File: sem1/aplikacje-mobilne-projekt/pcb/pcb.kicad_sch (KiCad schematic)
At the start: 26 parts, among them J1 Conn_01x20_Female, J2 Conn_01x20_Female, J3 Conn_01x10_Male, Q1 IRF540N, Q10 IRF540N, Q11 IRF540N, Q12 IRF540N, Q13 IRF540N, Q2 IRF540N, Q3 IRF540N, Q4 IRF540N, Q5 IRF540N, Q6 IRF540N, Q7 IRF540N, Q8 IRF540N, Q9 IRF540N, U1 IRF9540N, U2 IRF9540N, U3 IRF9540N, U4 IRF9540N

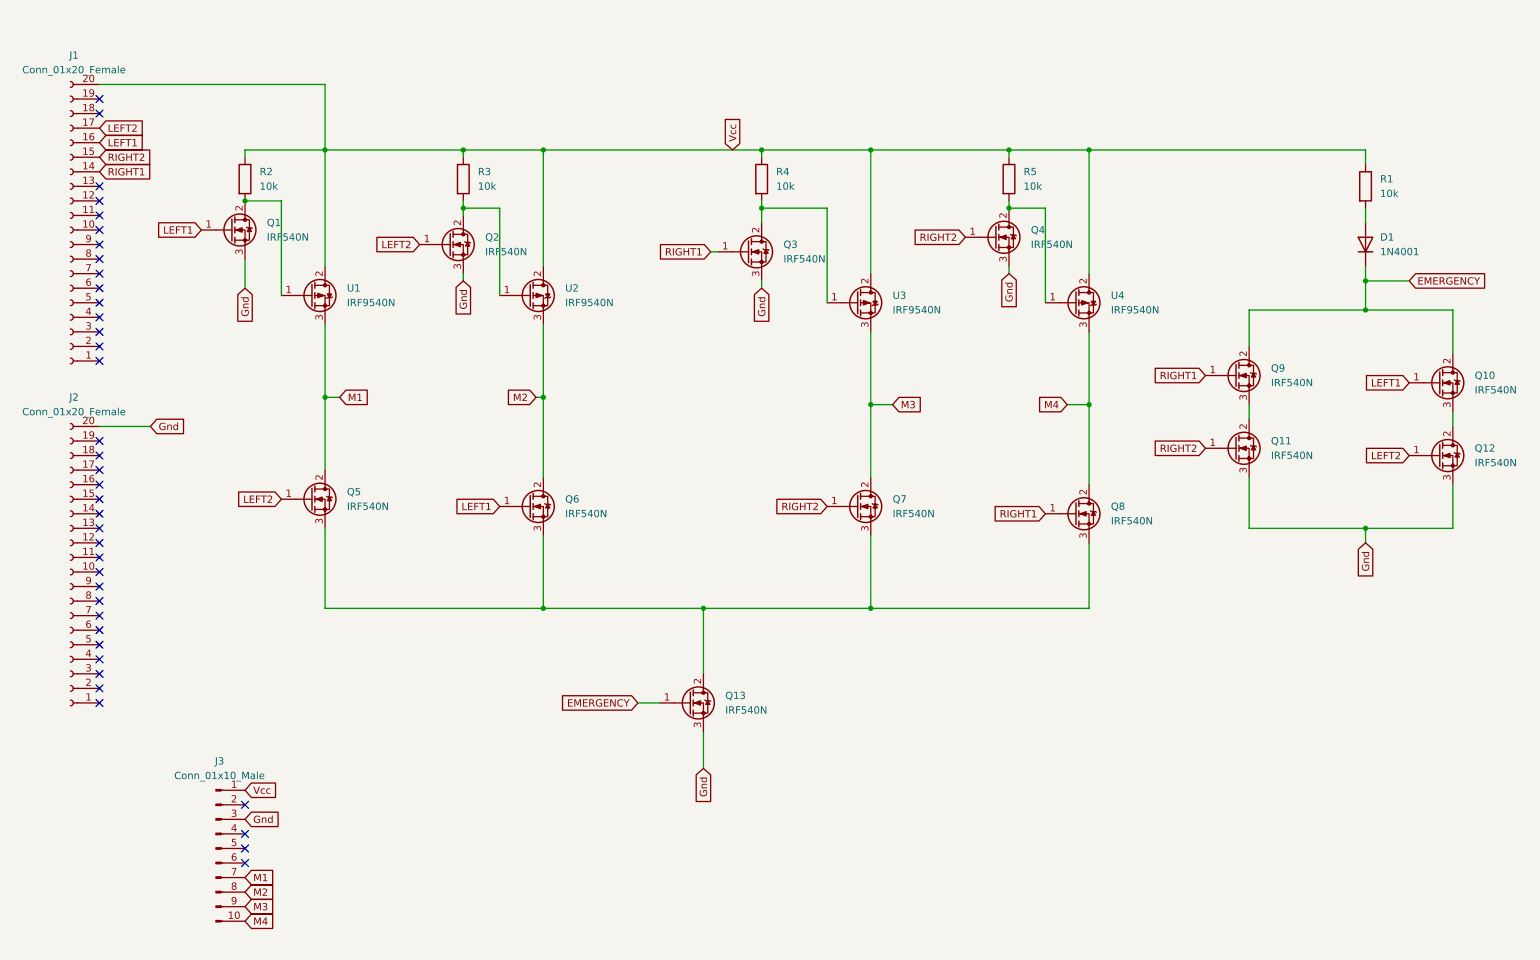
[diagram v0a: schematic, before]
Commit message: this pcb one actually works
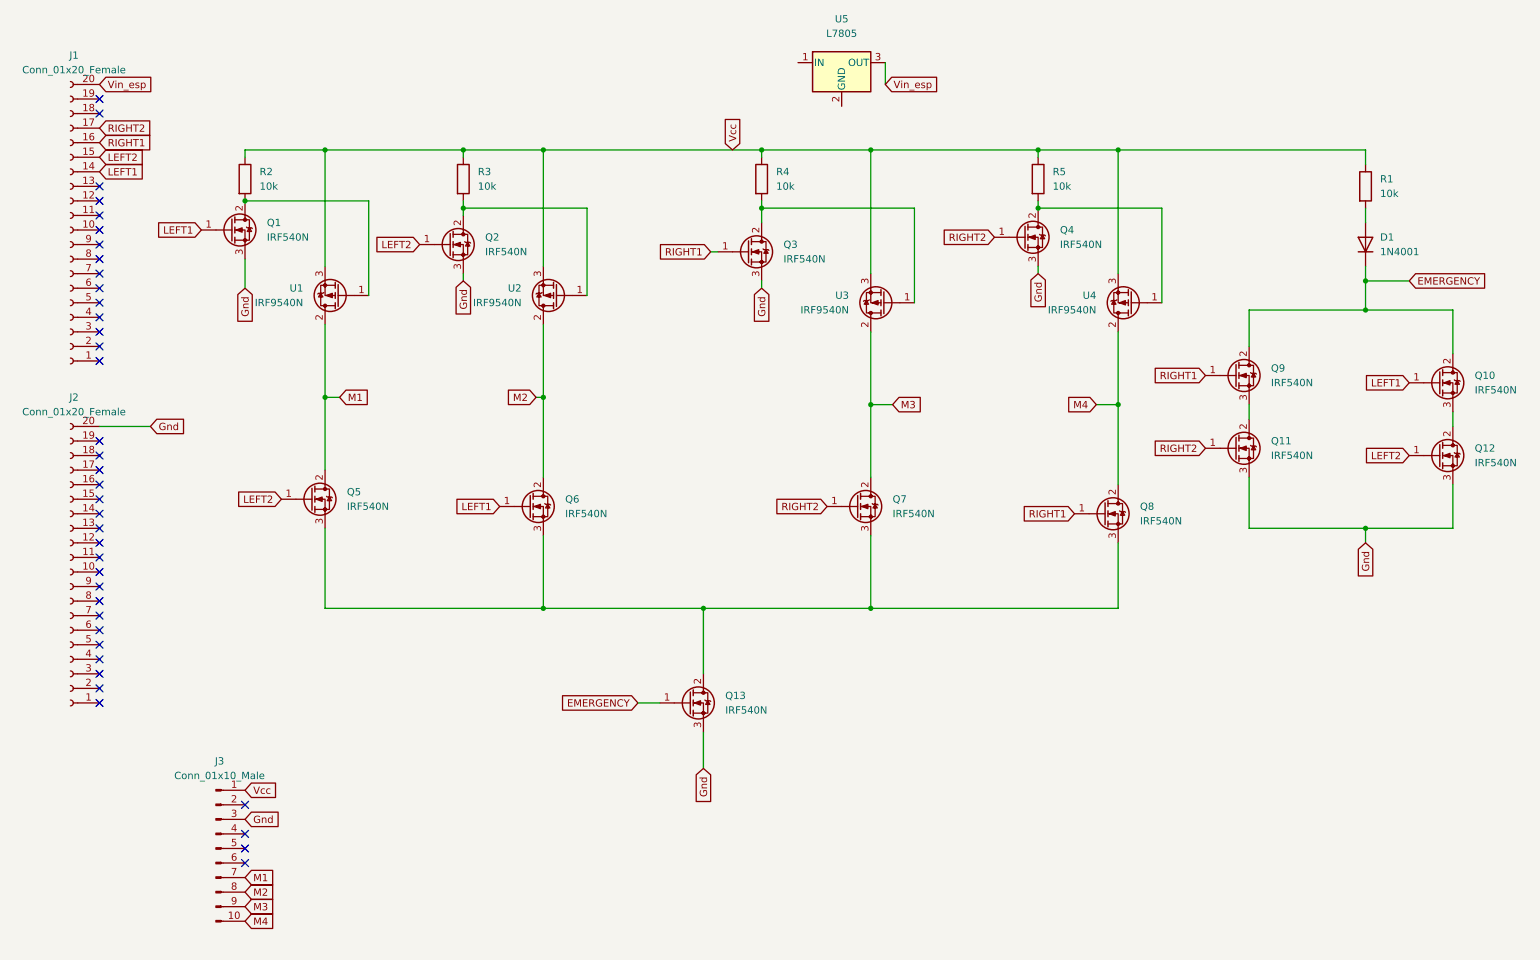
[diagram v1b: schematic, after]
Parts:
- added U5: L7805, symbol Regulator_Linear:L7805
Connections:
- net LEFT1: now also J1.14 (Pin_14); no longer J1.16 (Pin_16)
- net LEFT2: now also J1.15 (Pin_15); no longer J1.17 (Pin_17)
- net M1: now also U1.2 (D); no longer U1.3 (S)
- net M2: now also U2.2 (D); no longer U2.3 (S)
- net M3: now also U3.2 (D); no longer U3.3 (S)
- net M4: now also U4.2 (D); no longer U4.3 (S)
- net RIGHT1: now also J1.16 (Pin_16); no longer J1.14 (Pin_14)
- net RIGHT2: now also J1.17 (Pin_17); no longer J1.15 (Pin_15)
- net Vcc: now also U1.3 (S), U2.3 (S), U3.3 (S), U4.3 (S); no longer J1.20 (Pin_20), U1.2 (D), U2.2 (D), U3.2 (D), U4.2 (D)
- new net Vin_esp: J1.20 (Pin_20), U5.3 (OUT)
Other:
- moved on the sheet: Q4, Q8, R5, U1, U2, U3, U4

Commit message: PCB near end
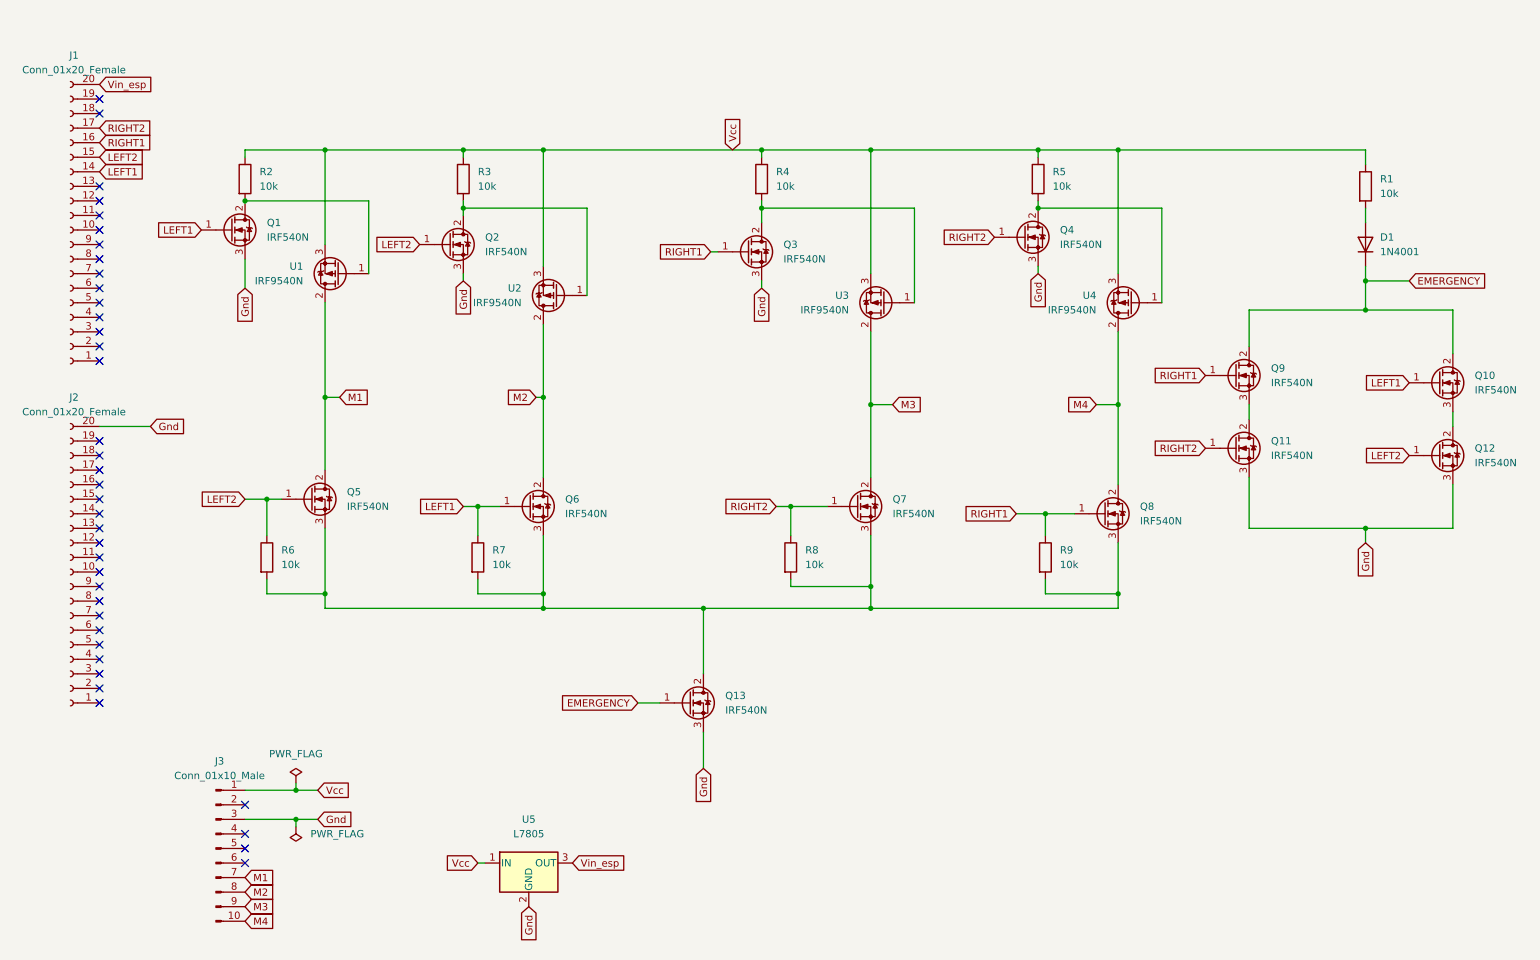
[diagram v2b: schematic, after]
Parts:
- added R6, R7, R8, R9: 10k, Resistor_THT:R_Axial_DIN0204_L3.6mm_D1.6mm_P7.62mm_Horizontal, symbol Device:R
- U5: footprint (none) -> Package_TO_SOT_THT:TO-220-3_Vertical
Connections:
- net Gnd: now also U5.2 (GND)
- net LEFT1: now also R7.1
- net LEFT2: now also R6.1
- net RIGHT1: now also R9.1
- net RIGHT2: now also R8.1
- net Vcc: now also U5.1 (IN)
- net at Q13.2 (D), Q5.3 (S), Q6.3 (S)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: now also R6.2, R7.2, R8.2, R9.2
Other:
- moved on the sheet: U1, U5

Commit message: pcb
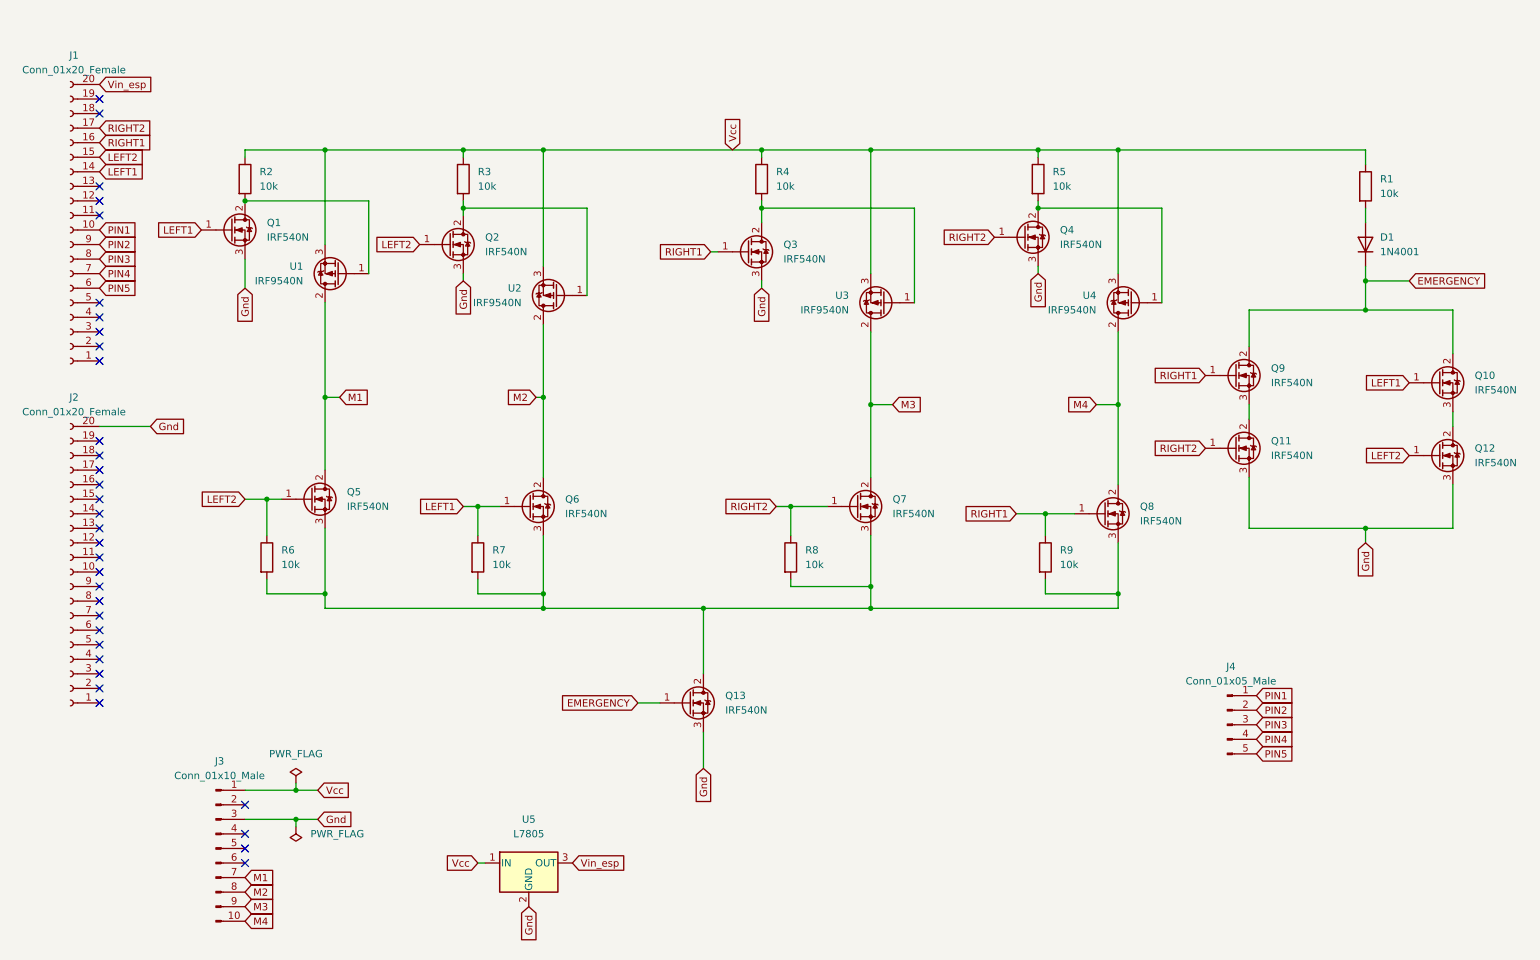
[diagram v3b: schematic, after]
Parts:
- added J4: Conn_01x05_Male, Connector_PinHeader_2.54mm:PinHeader_1x05_P2.54mm_Vertical, symbol Connector:Conn_01x05_Male
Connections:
- net PIN1: now reaches J1.10 (Pin_10)
- net PIN1: now also J4.1 (Pin_1)
- net PIN5: now reaches J1.6 (Pin_6)
- net PIN5: now also J4.5 (Pin_5)
- net PIN4: now reaches J1.7 (Pin_7)
- net PIN4: now also J4.4 (Pin_4)
- net PIN3: now reaches J1.8 (Pin_8)
- net PIN3: now also J4.3 (Pin_3)
- net PIN2: now reaches J1.9 (Pin_9)
- net PIN2: now also J4.2 (Pin_2)
- no-connect marks 38 -> 33
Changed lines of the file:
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@@
   (no_connect (at 26.67 110.49))
   (no_connect (at 26.67 53.34))
-  (no_connect (at 26.67 66.04))
   (no_connect (at 26.67 115.57))
   (no_connect (at 26.67 97.79))
@@
   (no_connect (at 26.67 135.89))
   (no_connect (at 26.67 107.95))
-  (no_connect (at 26.67 58.42))
   (no_connect (at 26.67 138.43))
   (no_connect (at 26.67 123.19))
   (no_connect (at 26.67 133.35))
   (no_connect (at 52.07 158.75))
-  (no_connect (at 26.67 60.96))
   (no_connect (at 26.67 118.11))
   (no_connect (at 26.67 95.25))
@@
   (no_connect (at 52.07 168.91))
   (no_connect (at 26.67 120.65))
-  (no_connect (at 26.67 63.5))
   (no_connect (at 26.67 76.2))
   (no_connect (at 26.67 81.28))
   (no_connect (at 26.67 140.97))
-  (no_connect (at 26.67 68.58))
   (no_connect (at 26.67 125.73))
   (no_connect (at 26.67 128.27))
@@
     )
   )
+  (global_label "PIN5" (shape input) (at 228.6 149.86 0) (fields_autoplaced)
+    (effects (font (size 1.27 1.27)) (justify left))
+    (property "Intersheet References" "${INTERSHEET_REFS}" (id 0) (at 235.4279 149.7806 0)
+      (effects (font (size 1.27 1.27)) (justify left) hide)
+    )
+  )
+  (global_label "PIN2" (shape input) (at 228.6 142.24 0) (fields_autoplaced)
+    (effects (font (size 1.27 1.27)) (justify left))
+    (property "Intersheet References" "${INTERSHEET_REFS}" (id 0) (at 235.4279 142.1606 0)
+      (effects (font (size 1.27 1.27)) (justify left) hide)
+    )
+  )
   (global_label "M3" (shape input) (at 165.1 88.9 0) (fields_autoplaced)
     (effects (font (size 1.27 1.27)) (justify left))
@@
     )
   )
+  (global_label "PIN3" (shape input) (at 26.67 63.5 0) (fields_autoplaced)
+    (effects (font (size 1.27 1.27)) (justify left))
+    (property "Intersheet References" "${INTERSHEET_REFS}" (id 0) (at 33.4979 63.4206 0)
+      (effects (font (size 1.27 1.27)) (justify left) hide)
+    )
+  )
   (global_label "LEFT2" (shape input) (at 26.67 45.72 0) (fields_autoplaced)
     (effects (font (size 1.27 1.27)) (justify left))
@@
     )
   )
+  (global_label "PIN1" (shape input) (at 26.67 58.42 0) (fields_autoplaced)
+    (effects (font (size 1.27 1.27)) (justify left))
+    (property "Intersheet References" "${INTERSHEET_REFS}" (id 0) (at 33.4979 58.3406 0)
+      (effects (font (size 1.27 1.27)) (justify left) hide)
+    )
+  )
   (global_label "Gnd" (shape input) (at 132.08 152.4 270) (fields_autoplaced)
     (effects (font (size 1.27 1.27)) (justify right))
@@
     )
   )
+  (global_label "PIN5" (shape input) (at 26.67 68.58 0) (fields_autoplaced)
+    (effects (font (size 1.27 1.27)) (justify left))
+    (property "Intersheet References" "${INTERSHEET_REFS}" (id 0) (at 33.4979 68.5006 0)
+      (effects (font (size 1.27 1.27)) (justify left) hide)
+    )
+  )
   (global_label "RIGHT1" (shape input) (at 26.67 43.18 0) (fields_autoplaced)
     (effects (font (size 1.27 1.27)) (justify left))
@@
     )
   )
+  (global_label "PIN1" (shape input) (at 228.6 139.7 0) (fields_autoplaced)
+    (effects (font (size 1.27 1.27)) (justify left))
+    (property "Intersheet References" "${INTERSHEET_REFS}" (id 0) (at 235.4279 139.6206 0)
+      (effects (font (size 1.27 1.27)) (justify left) hide)
+    )
+  )
   (global_label "LEFT1" (shape input) (at 255.27 85.09 180) (fields_autoplaced)
     (effects (font (size 1.27 1.27)) (justify right))
@@
     )
   )
+  (global_label "PIN2" (shape input) (at 26.67 60.96 0) (fields_autoplaced)
+    (effects (font (size 1.27 1.27)) (justify left))
+    (property "Intersheet References" "${INTERSHEET_REFS}" (id 0) (at 33.4979 60.8806 0)
+      (effects (font (size 1.27 1.27)) (justify left) hide)
+    )
+  )
+  (global_label "PIN3" (shape input) (at 228.6 144.78 0) (fields_autoplaced)
+    (effects (font (size 1.27 1.27)) (justify left))
+    (property "Intersheet References" "${INTERSHEET_REFS}" (id 0) (at 235.4279 144.7006 0)
+      (effects (font (size 1.27 1.27)) (justify left) hide)
+    )
+  )
   (global_label "LEFT1" (shape input) (at 90.17 106.68 180) (fields_autoplaced)
     (effects (font (size 1.27 1.27)) (justify right))
@@
     (effects (font (size 1.27 1.27)) (justify left))
     (property "Intersheet References" "${INTERSHEET_REFS}" (id 0) (at 35.7355 40.5606 0)
+      (effects (font (size 1.27 1.27)) (justify left) hide)
+    )
+  )
+  (global_label "PIN4" (shape input) (at 26.67 66.04 0) (fields_autoplaced)
+    (effects (font (size 1.27 1.27)) (justify left))
+    (property "Intersheet References" "${INTERSHEET_REFS}" (id 0) (at 33.4979 65.9606 0)
+      (effects (font (size 1.27 1.27)) (justify left) hide)
+    )
+  )
+  (global_label "PIN4" (shape input) (at 228.6 147.32 0) (fields_autoplaced)
+    (effects (font (size 1.27 1.27)) (justify left))
+    (property "Intersheet References" "${INTERSHEET_REFS}" (id 0) (at 235.4279 147.2406 0)
       (effects (font (size 1.27 1.27)) (justify left) hide)
     )
@@
     (pin "1")
     (pin "2")
+  )
+  (symbol (lib_id "Connector:Conn_01x05_Male") (at 223.52 144.78 0) (unit 1)
+    (in_bom yes) (on_board yes) (fields_autoplaced)
+    (property "Reference" "J4" (id 0) (at 224.155 134.62 0))
+    (property "Value" "Conn_01x05_Male" (id 1) (at 224.155 137.16 0))
+    (property "Footprint" "Connector_PinHeader_2.54mm:PinHeader_1x05_P2.54mm_Vertical" (id 2) (at 223.52 144.78 0)
+      (effects (font (size 1.27 1.27)) hide)
+    )
+    (property "Datasheet" "~" (id 3) (at 223.52 144.78 0)
+      (effects (font (size 1.27 1.27)) hide)
+    )
+    (pin "1")
+    (pin "2")
+    (pin "3")
+    (pin "4")
+    (pin "5")
   )
   (symbol (lib_id "Transistor_FET:IRF540N") (at 187.96 59.69 0) (unit 1)
@@
       (reference "J3") (unit 1) (value "Conn_01x10_Male") (footprint "Connector_PinHeader_2.54mm:PinHeader_1x10_P2.54mm_Vertical")
     )
+    (path "/121ea4be-1933-4777-9ef0-8bd15d27e07d"
+      (reference "J4") (unit 1) (value "Conn_01x05_Male") (footprint "Connector_PinHeader_2.54mm:PinHeader_1x05_P2.54mm_Vertical")
+    )
     (path "/0a301908-afe3-461a-8352-30d5741534ec"
